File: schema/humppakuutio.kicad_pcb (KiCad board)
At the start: 2 copper layers, 21 parts, among them P1 CONN_01X05, U1 TL074, U2 WT32

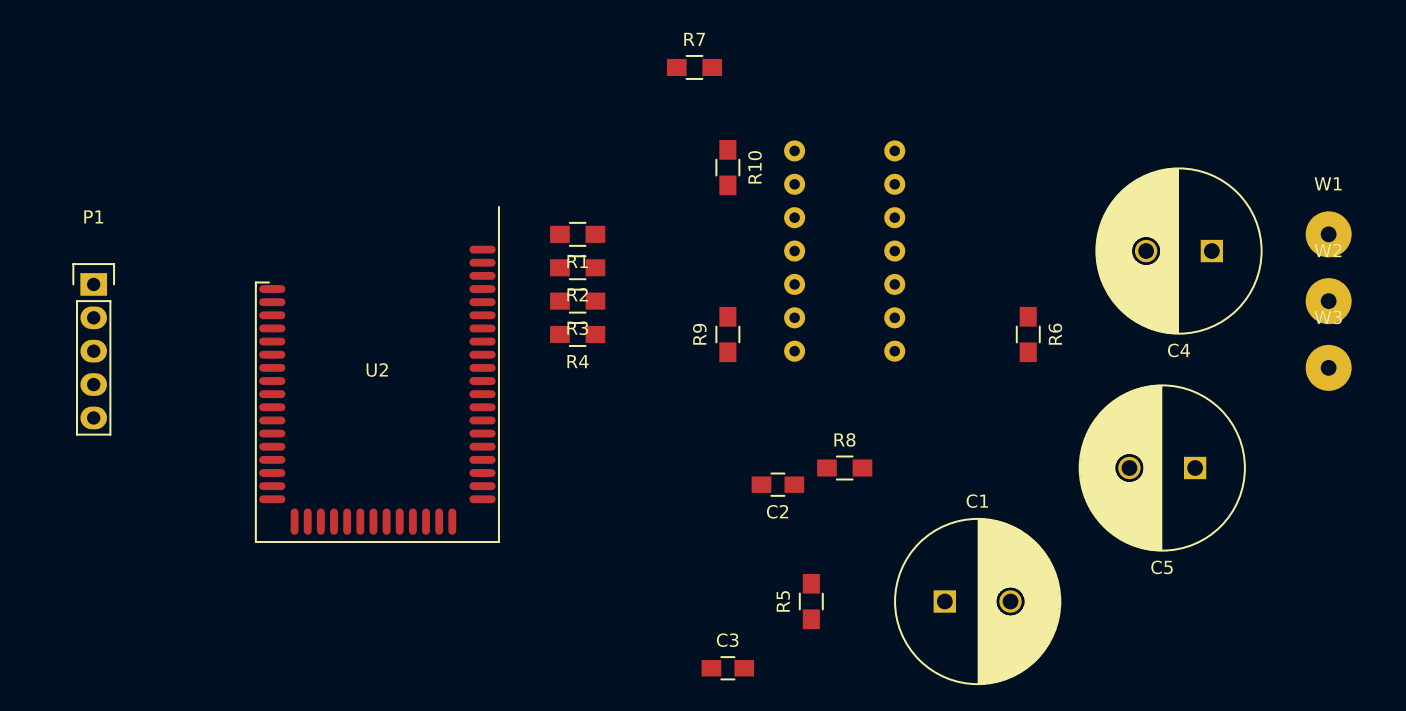
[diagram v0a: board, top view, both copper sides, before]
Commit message: HW ready for making
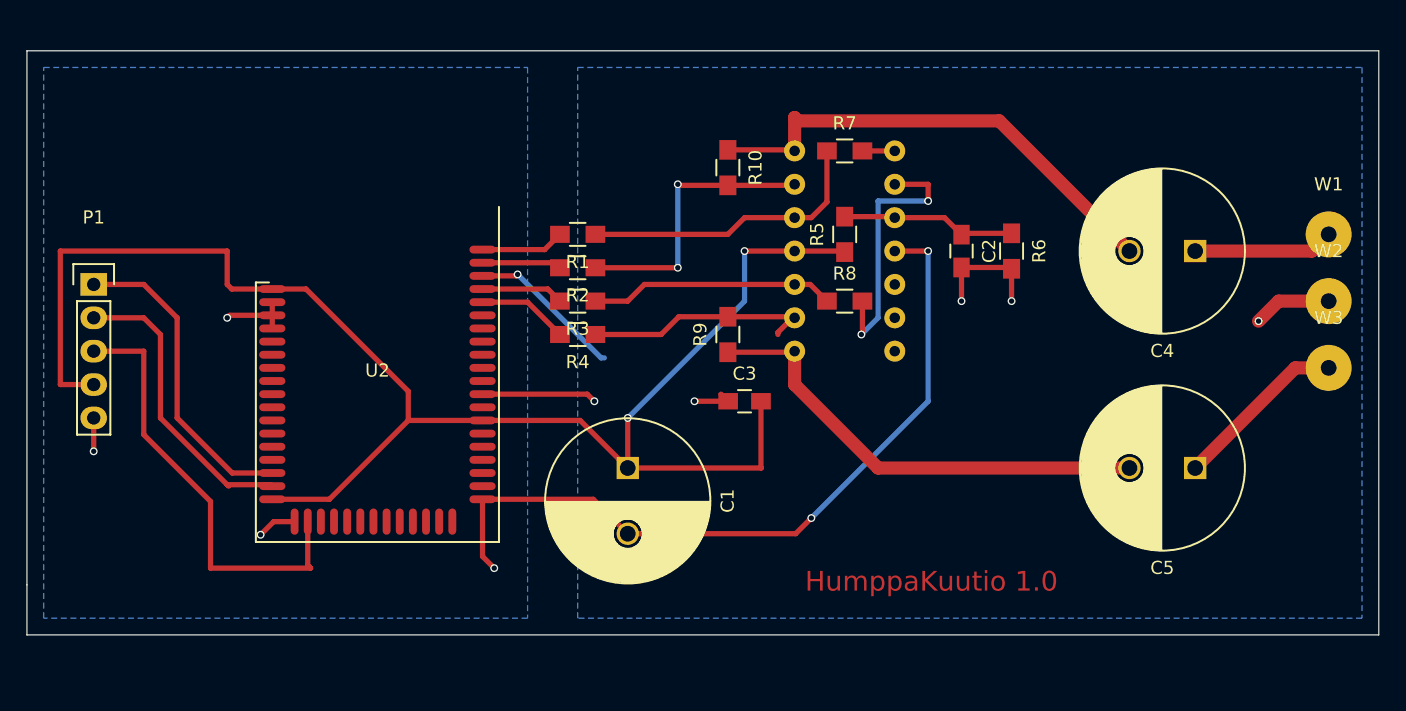
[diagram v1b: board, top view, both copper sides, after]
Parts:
- moved R5 28.1 mm to (184.2, 88.9)
- moved C1 26.2 mm to (167.6, 106.7), turned to 270 degrees
- moved C2 22.6 mm to (193.0, 90.2), turned to 270 degrees
- moved C3 20.4 mm to (176.5, 101.6)
- moved R7 13.1 mm to (184.2, 82.5)
- moved R8 12.7 mm to (184.2, 94.0)
- moved R6 6.48 mm to (196.8, 90.2)
- moved C4 1.27 mm to (210.8, 90.2)
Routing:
- net VCC: track 0.00 -> 121.4 mm, vias 0 -> 2
- net GNDD: track 0.00 -> 70.1 mm, vias 0 -> 6
- net GNDA: track 0.00 -> 38.8 mm, vias 0 -> 6
- net Net-(C4-Pad2): track 0.00 -> 37.3 mm
- net Net-(C5-Pad2): track 0.00 -> 35.8 mm
- net Net-(P1-Pad3): track 0.00 -> 33.7 mm
- net Net-(P1-Pad1): track 0.00 -> 24.0 mm
- net VCOM: track 0.00 -> 23.3 mm, vias 0 -> 2
- net Net-(P1-Pad2): track 0.00 -> 22.8 mm
- net Net-(R1-Pad1): track 0.00 -> 22.5 mm
- net Net-(R10-Pad2): track 0.00 -> 21.6 mm, vias 0 -> 2
- net Net-(R3-Pad1): track 0.00 -> 18.7 mm
- net Net-(R4-Pad1): track 0.00 -> 17.5 mm
- net Net-(C5-Pad1): track 0.00 -> 13.3 mm
- net Net-(C2-Pad1): track 0.00 -> 13.2 mm
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- added copper zone on B.Cu, net GNDA
- added copper zone on B.Cu, net GNDD
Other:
- board outline added: 102.9 x 44.4 mm
- net class Default: trace_width 0.25 -> 0.4
- rule trace_min: 0.25 -> 0.4
- board text added: "HumppaKuutio 1.0"
